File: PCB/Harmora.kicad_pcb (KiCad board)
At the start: 2 copper layers, 355.8 x 282 mm, 5 parts, among them U2 SS49E

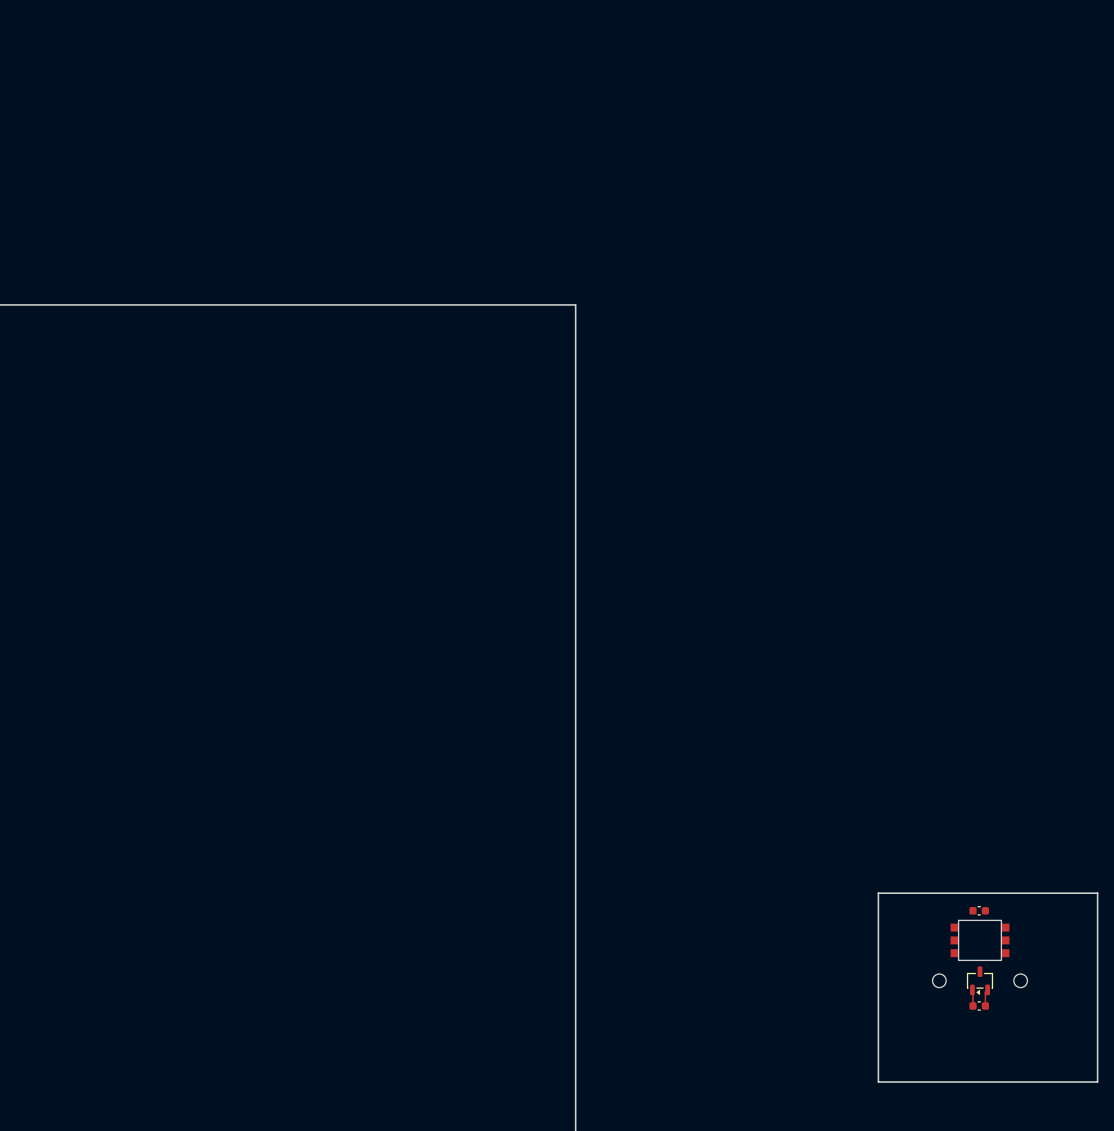
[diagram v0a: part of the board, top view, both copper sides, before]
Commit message: new schematics
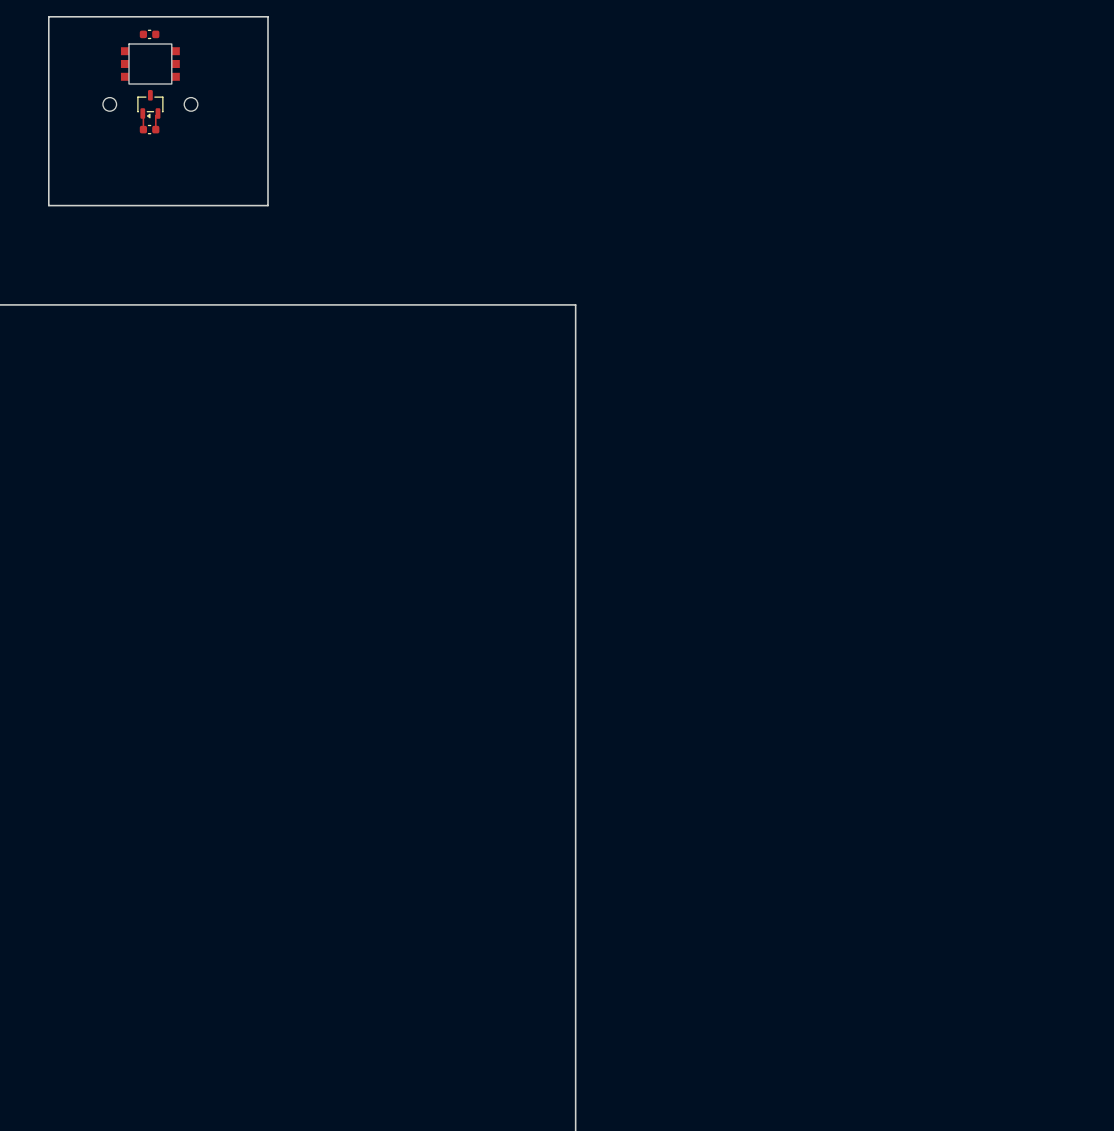
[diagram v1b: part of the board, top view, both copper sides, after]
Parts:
- moved C1 150.8 mm to (-79.1, -83.3)
- moved REF** 150.8 mm to (-79.0, -91.5)
- moved REF** 150.8 mm to (-79.1, -95.2)
- moved REF** 150.8 mm to (-79.0, -86.5)
- moved U2 150.8 mm to (-79.0, -86.5)
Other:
- board size 355.8 x 282 mm -> 290.6 x 318.1 mm
